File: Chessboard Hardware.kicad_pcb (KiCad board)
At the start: 2 copper layers, 200 x 200 mm, 100 parts, among them J1 Conn_01x04_Pin

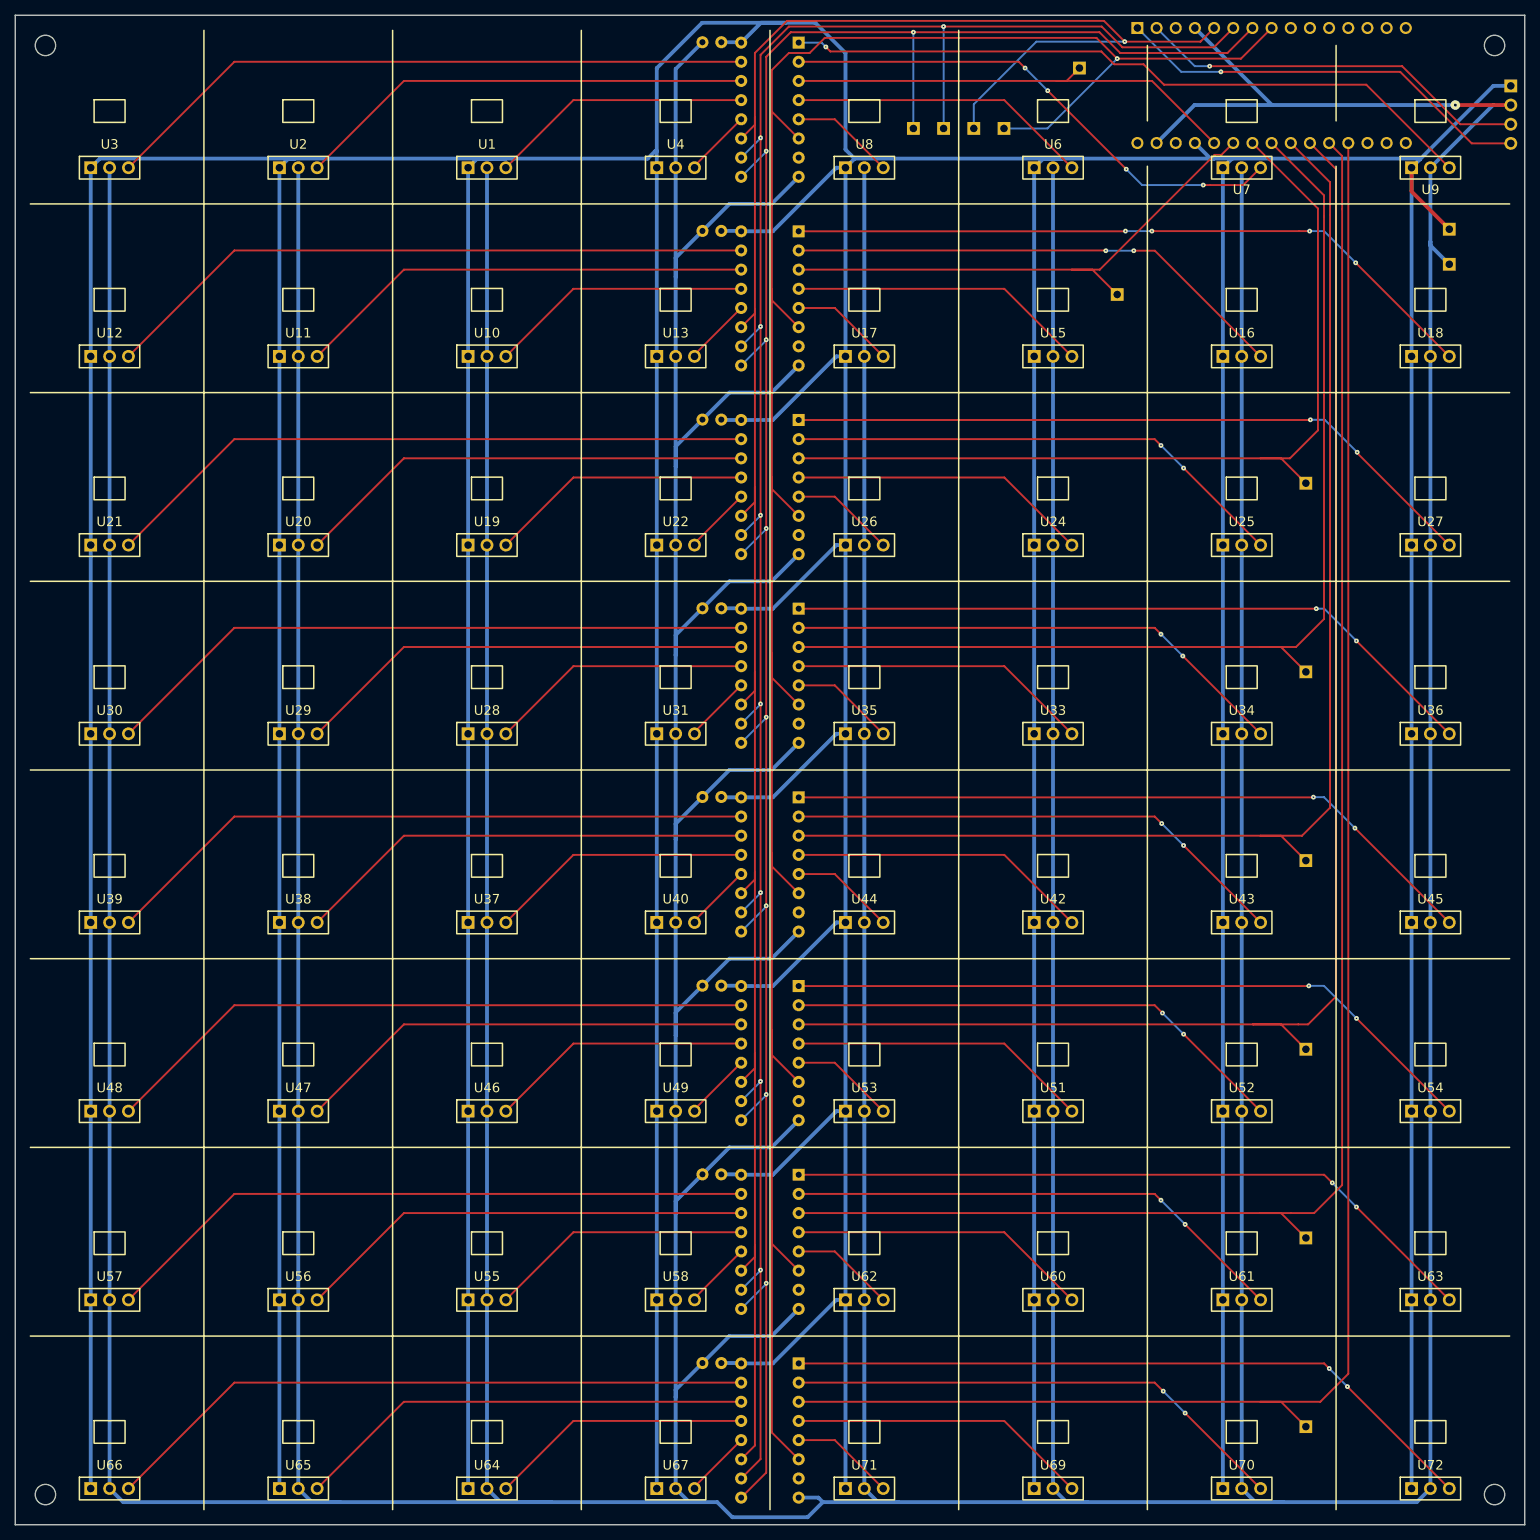
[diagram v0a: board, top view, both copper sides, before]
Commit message: Ground plane
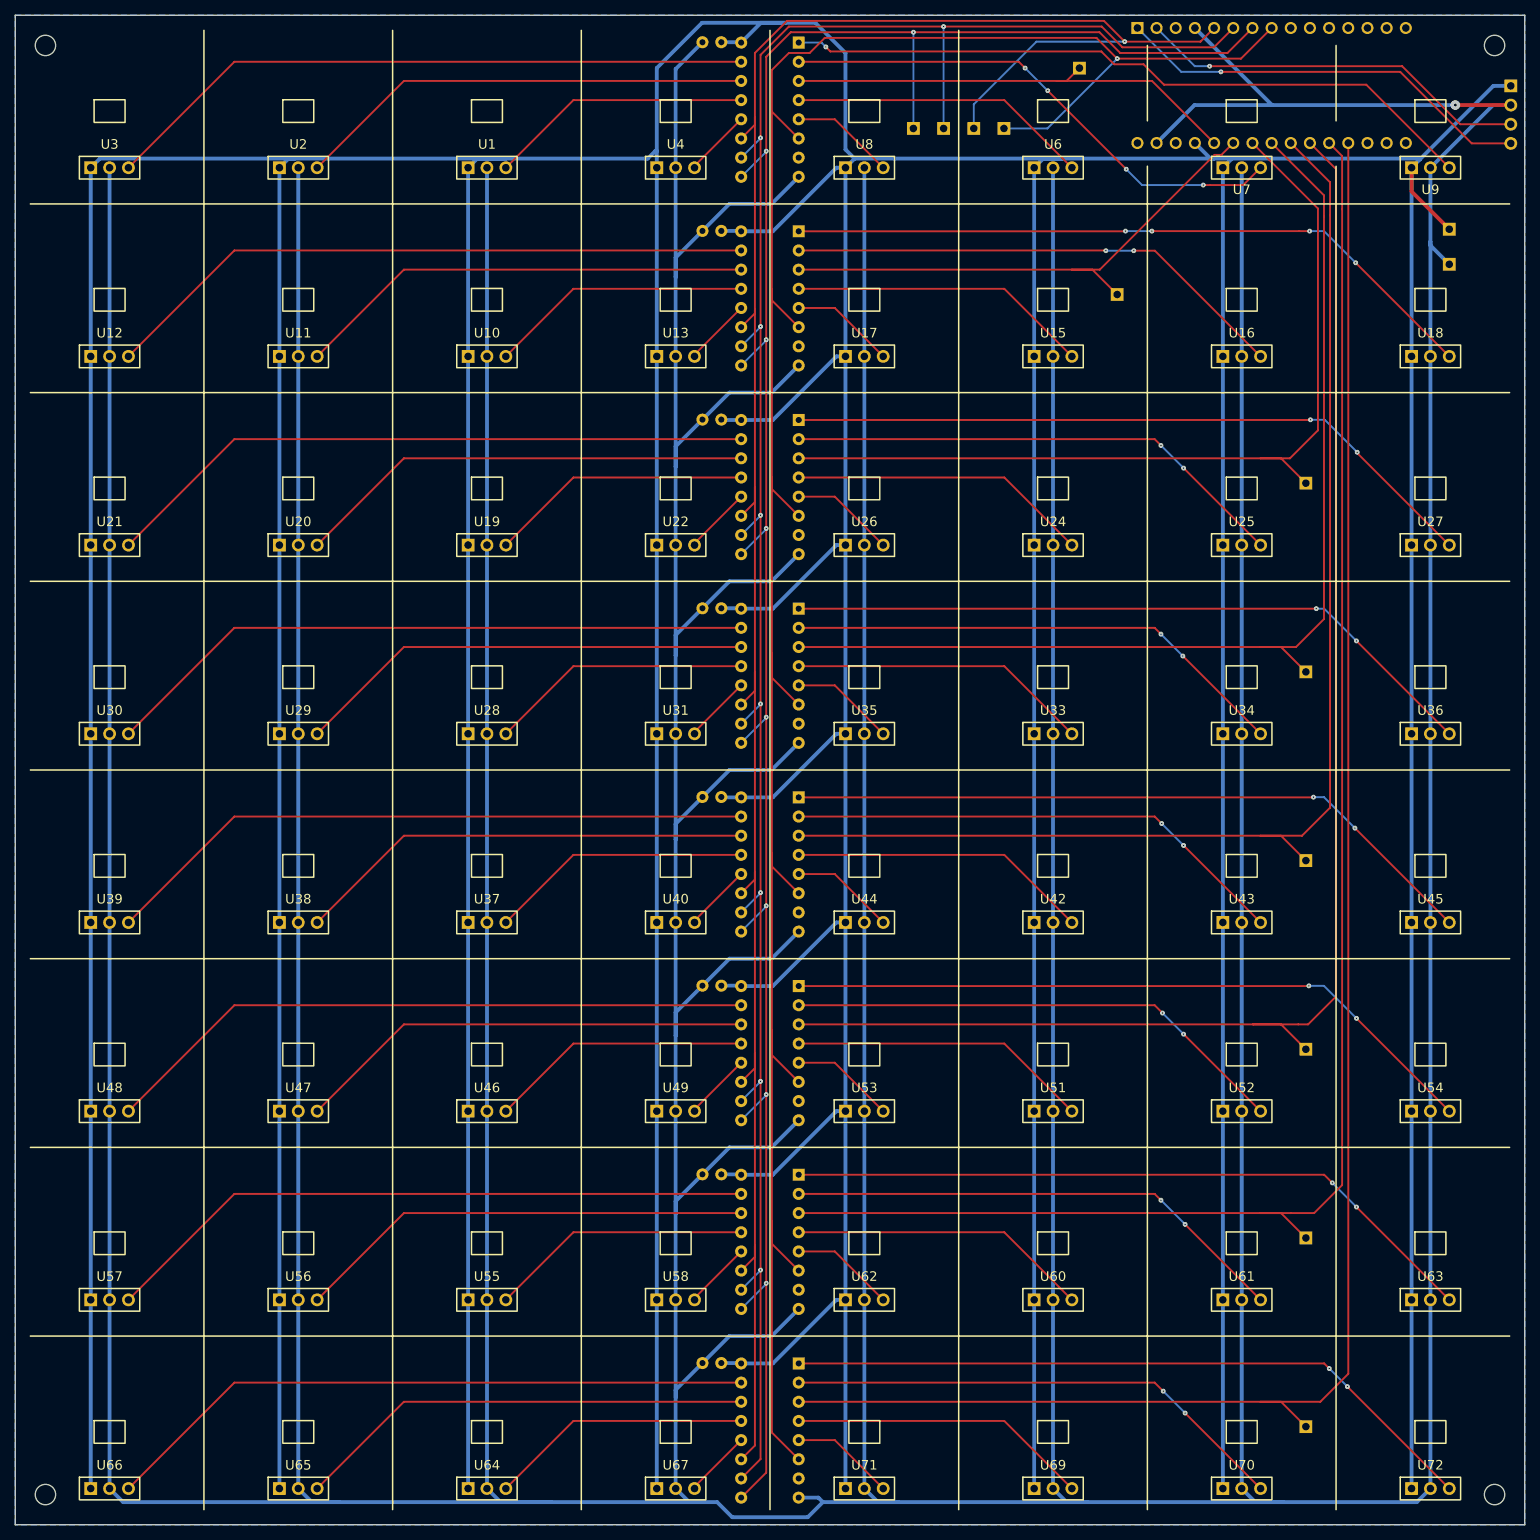
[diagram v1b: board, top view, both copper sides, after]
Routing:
- added copper zone on B.Cu, net GND
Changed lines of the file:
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@@
 		(net 100)
 	)
+	(zone
+		(net 12)
+		(net_name "GND")
+		(layer "B.Cu")
+		(hatch edge 0.5)
+		(connect_pads
+			(clearance 0.508)
+		)
+		(min_thickness 0.25)
+		(filled_areas_thickness no)
+		(fill yes
+			(thermal_gap 0.5)
+			(thermal_bridge_width 0.5)
+		)
+		(polygon
+			(pts
+				(xy 50 50) (xy 250 50.000001) (xy 250 250) (xy 50 250)
+			)
+		)
+	)
 )
